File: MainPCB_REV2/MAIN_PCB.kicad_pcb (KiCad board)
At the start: 2 copper layers, 82 x 99.5 mm, 73 parts, among them U1 INA226, U2 DRV8871DDA, U3 INA226

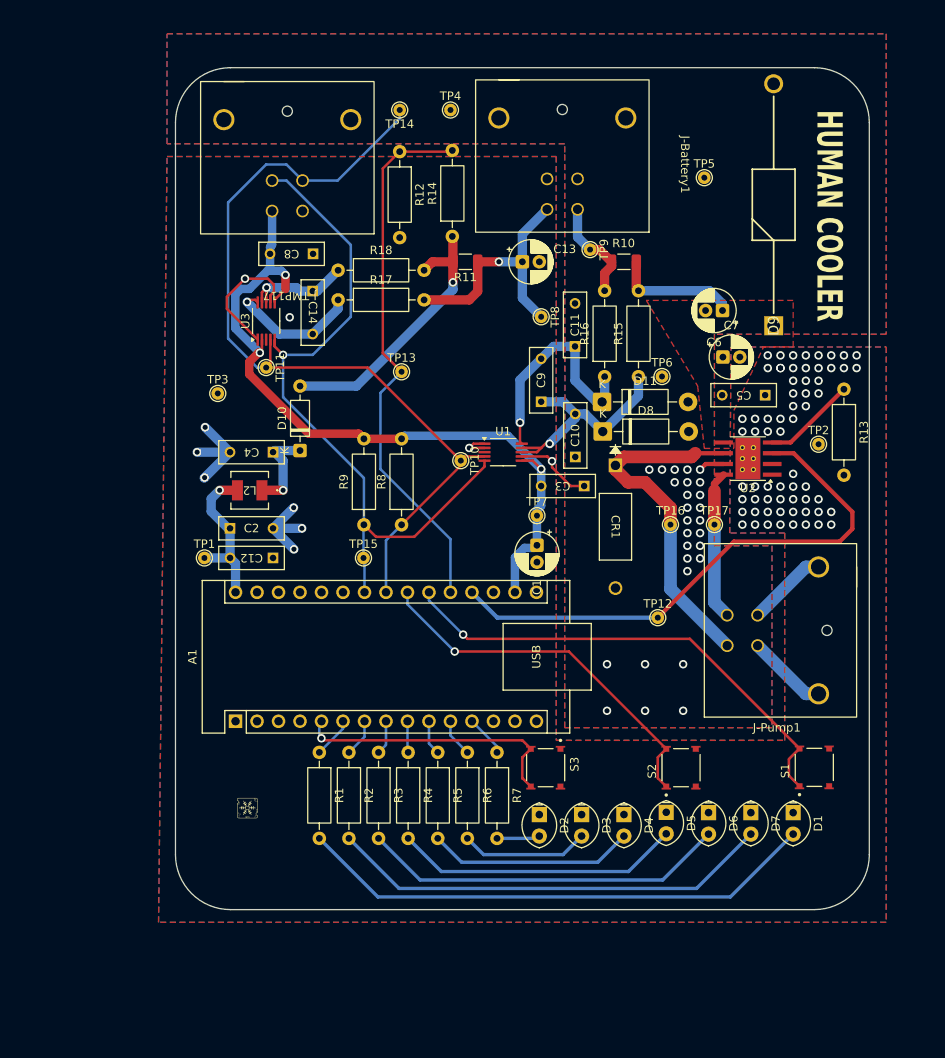
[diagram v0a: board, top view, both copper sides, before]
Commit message: 3/23
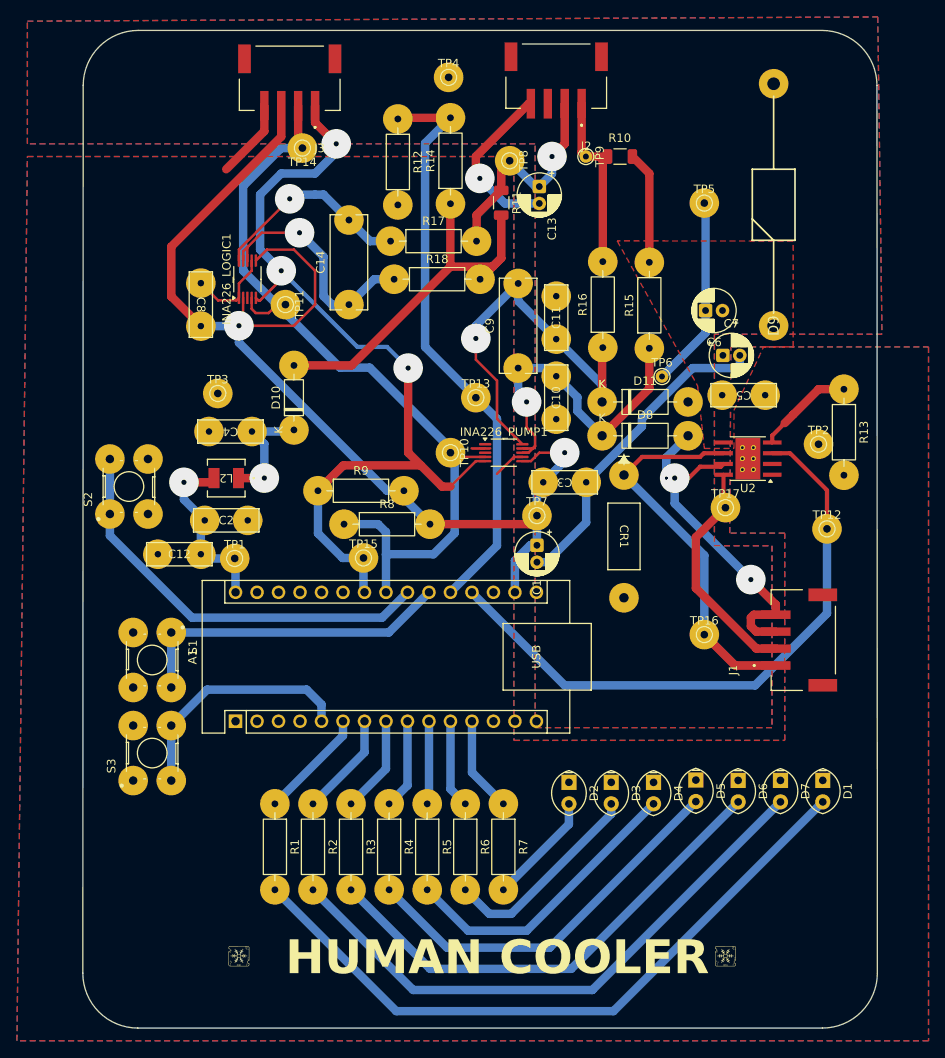
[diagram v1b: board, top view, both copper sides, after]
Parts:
- removed J-Battery1, J-Pump1, J-TMP117: 861-004-213R00Y, 861.preety:861-004-213R00Y
- removed U1, U3: INA226, Package_SO:VSSOP-10_3x3mm_P0.5mm
- added G***: LOGO, LOGO.preety:P16logo, F.Cu at (165.0, 151.5)
- added INA226_LOGIC1: INA226, Package_SO:VSSOP-10_3x3mm_P0.5mm, F.Cu at (108.5, 71.5)
- added INA226_PUMP1: INA226, Package_SO:VSSOP-10_3x3mm_P0.5mm, F.Cu at (138.8, 92.0)
- added J1: 12V DC PUMP, S4B_PH_SM4_TB:JST_S4B-PH-SM4-TB, F.Cu at (173.7, 114.2)
- added J2: 12.8V LFP BATTERY, S4B_PH_SM4_TB:JST_S4B-PH-SM4-TB, F.Cu at (145.0, 48.0)
- added J3: TMP117s, S4B_PH_SM4_TB:JST_S4B-PH-SM4-TB, F.Cu at (113.5, 48.2)
- C14, C9: footprint CAP_BF01:CAP_BF01_AVX -> Capacitor_THT:C_Rect_L11.0mm_W4.2mm_P10.00mm_MKT
- S1: value TL3315NF250Q -> + BUTTON; footprint TL3315NF250Q:SW_TL3315NF250Q -> B3F_1000:SW_B3F-1000
- S2: value TL3315NF250Q -> - BUTTON; footprint TL3315NF250Q:SW_TL3315NF250Q -> B3F_1000:SW_B3F-1000
- S3: value TL3315NF250Q -> AUTO BUTTON; footprint TL3315NF250Q:SW_TL3315NF250Q -> B3F_1000:SW_B3F-1000
- moved S1 79.3 mm to (97.2, 116.5), turned to -90 degrees
- moved S2 73.2 mm to (94.5, 96.0)
- moved S3 46.5 mm to (97.2, 127.5), turned to 90 degrees
- moved TP12 22.6 mm to (177.0, 101.0)
- moved TP8 18.8 mm to (139.5, 57.5)
- moved G*** 17.5 mm to (107.5, 151.5)
- moved C8 13.7 mm to (103.0, 72.0), turned to -90 degrees
- moved C12 13.6 mm to (97.9, 104.0), turned to 0 degrees
- moved TP16 13.6 mm to (162.5, 113.5)
- moved R10 12.4 mm to (152.5, 57.0)
- moved TP14 12.3 mm to (115.0, 56.0)
- moved TP9 11.0 mm to (148.5, 57.0)
- moved R17 9.31 mm to (125.4, 67.0)
- moved TP13 9.30 mm to (135.5, 85.5)
- moved C13 9.12 mm to (143.0, 60.5), turned to -90 degrees
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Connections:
- net +BATT renamed Net-(D10-A)
- net DRV renamed Net-(U2-OUT1)
- net RTN renamed Net-(U2-OUT2)
- net Vdrive renamed Net-(D9-K)
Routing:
- net +3.3V: track 89.9 -> 136.1 mm, vias 3 -> 2
- net GNDPWR: track 22.2 -> 64.1 mm, vias 27 -> 5
- net GND: track 51.3 -> 83.6 mm, vias 74 -> 1
- net Net-(D11-K): track 27.1 -> 47.9 mm
- net SCL: track 84.1 -> 103.7 mm, vias 1 -> 3
- net Net-(D1-A): track 61.9 -> 80.9 mm
- net Net-(A1-A2): track 57.5 -> 38.9 mm, vias 1 -> 0
- net Net-(D7-A): track 52.6 -> 69.4 mm
- net Net-(INA226_LOGIC1-Vbus): track 13.4 -> 29.1 mm
- net Net-(D6-A): track 43.3 -> 57.8 mm
- net Net-(D10-A): track 32.9 -> 45.8 mm, vias 1 -> 0
- net Net-(D8-K): track 27.8 -> 40.3 mm
- net Net-(D5-A): track 34.0 -> 46.2 mm
- net Net-(D4-A): track 24.4 -> 35.0 mm
- net Net-(U2-OUT2): track 17.7 -> 27.3 mm
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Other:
- board size 82 x 99.5 mm -> 93.9 x 117.9 mm
